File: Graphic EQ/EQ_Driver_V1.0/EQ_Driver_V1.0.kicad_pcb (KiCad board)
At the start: 2 copper layers, 127 x 57.2 mm, 35 parts, among them Q1 MPSA63, Q2 MPSA70, Q3 MPSA70, Q4 MPSA20

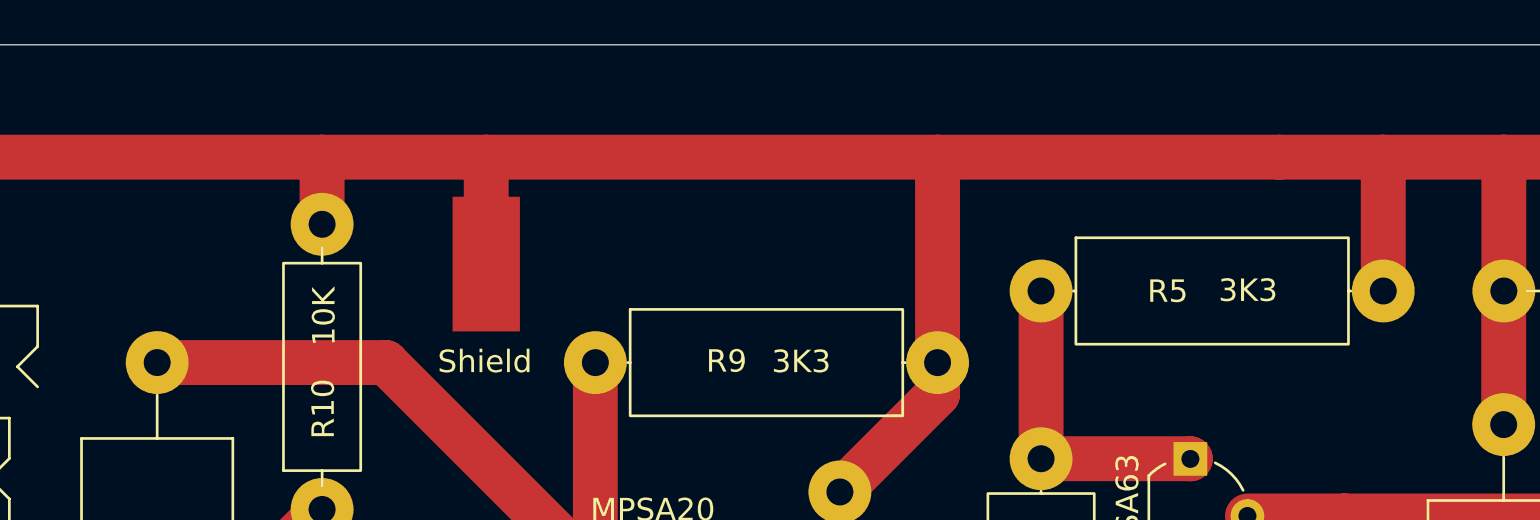
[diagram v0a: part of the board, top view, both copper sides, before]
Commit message: Preamp Progress, and Custom Footprint Library
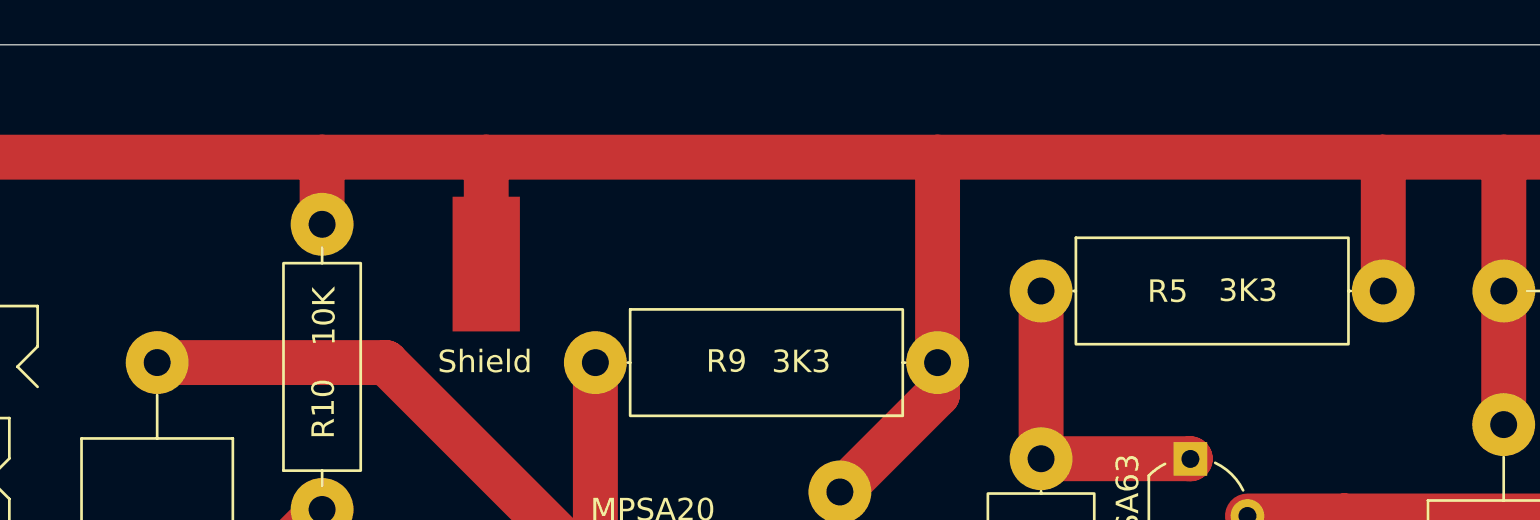
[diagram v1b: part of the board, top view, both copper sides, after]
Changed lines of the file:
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@@
-	)
-	(segment
-		(start 153.72 70.38)
-		(end 168.94 70.38)
-		(width 2)
-		(layer "F.Cu")
-		(net 2)
 	)
 	(segment
@@
 	)
 	(segment
-		(start 168.94 70.38)
+		(start 153.72 70.38)
 		(end 173.55 70.38)
 		(width 2)
@@
 		(width 2)
 		(layer "F.Cu")
-		(net 6)
-	)
-	(segment
-		(start 118.9671 79.53)
-		(end 118.9643 79.5272)
-		(width 2)
-		(layer "F.Cu")
